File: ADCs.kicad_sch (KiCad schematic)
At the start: 4 parts, among them U3 ADS7828, U4 ADS7828

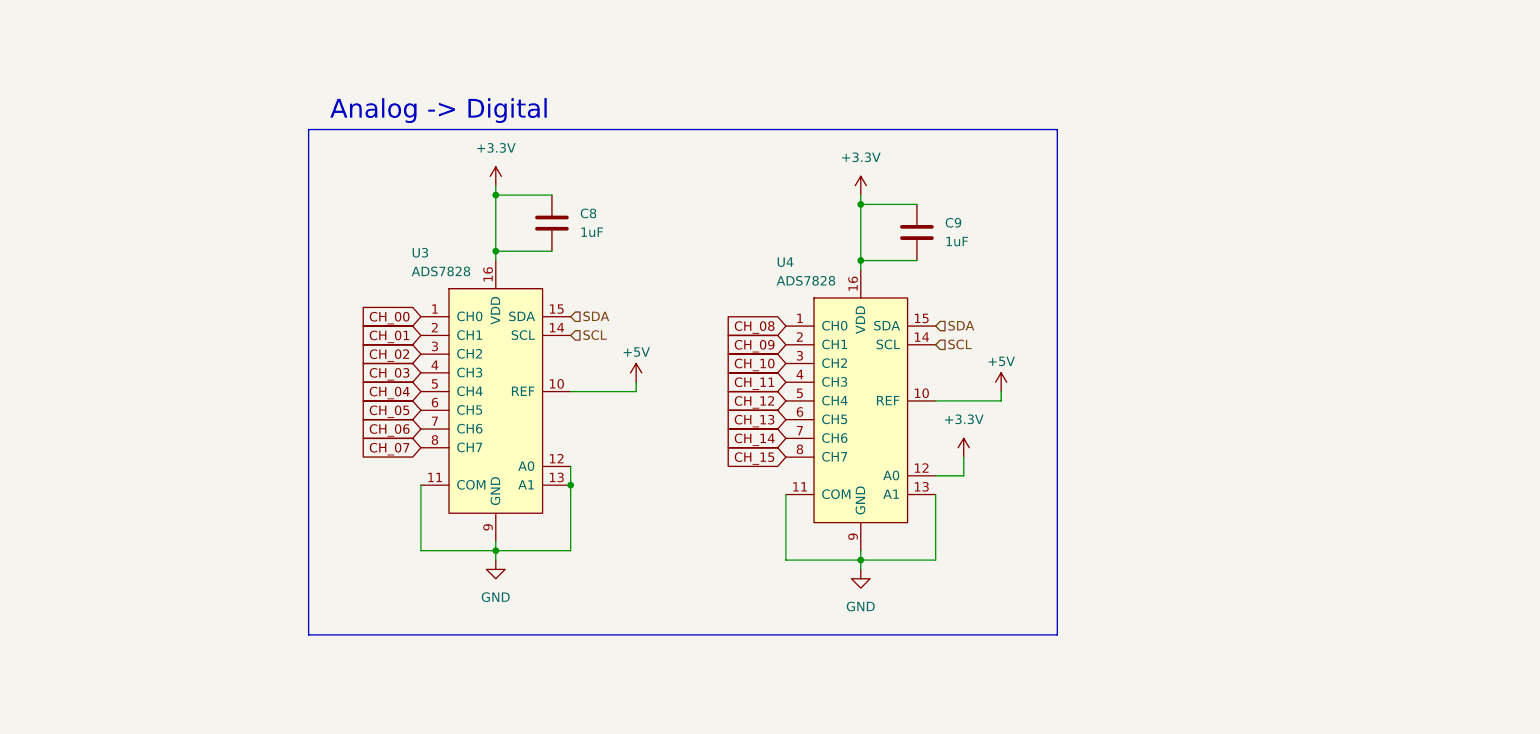
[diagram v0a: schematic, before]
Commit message: layout🏄‍♂️
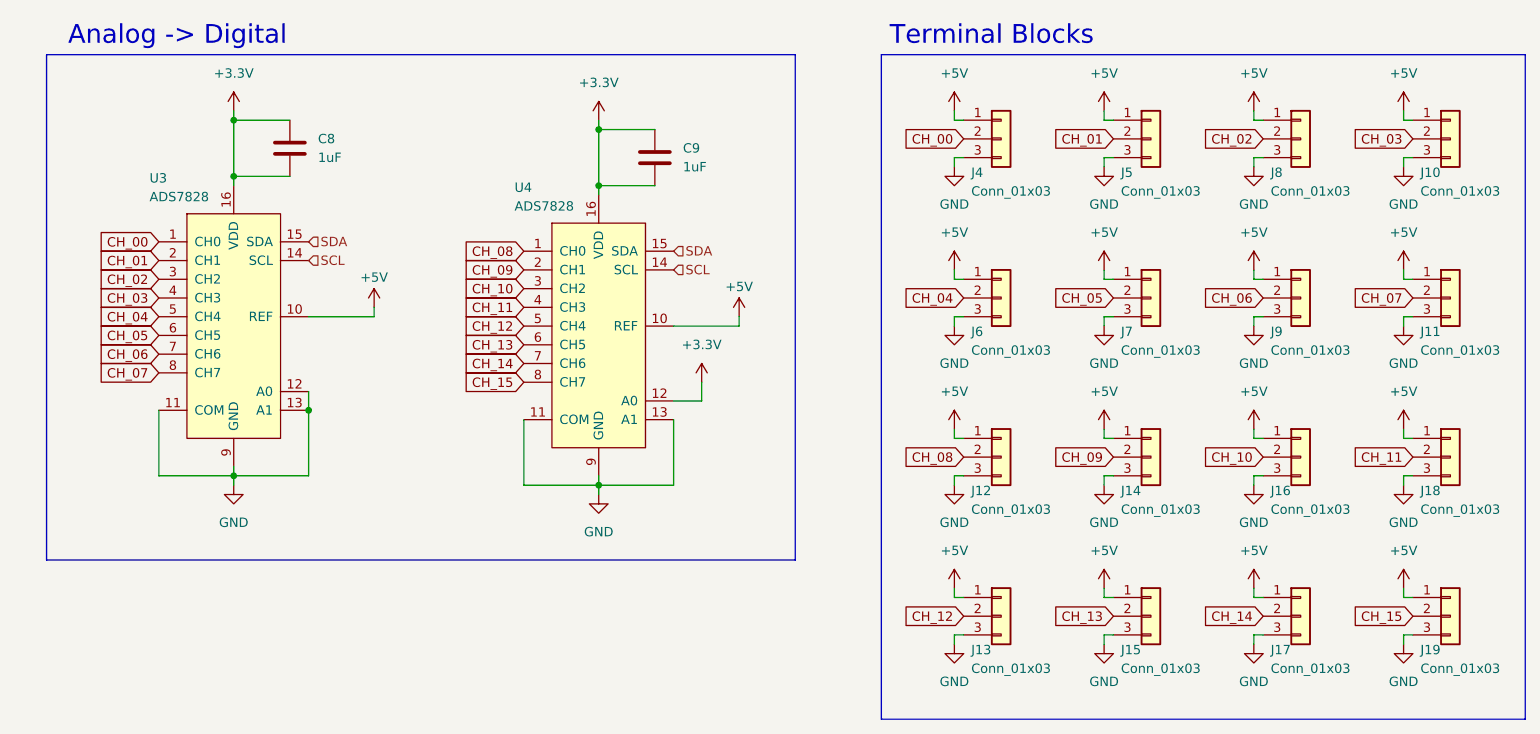
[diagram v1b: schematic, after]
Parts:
- added J10, J11, J12, J13, J14, J15, J16, J17, J18, J19, J4, J5, J6, J7, J8, J9: Conn_01x03, TerminalBlock_Phoenix:TerminalBlock_Phoenix_MPT-0,5-3-2.54_1x03_P2.54mm_Horizontal, symbol Connector_Generic:Conn_01x03
- C8, C9: footprint (none) -> Capacitor_SMD:C_0603_1608Metric
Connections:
- net +5V: now also J10.1 (Pin_1), J11.1 (Pin_1), J12.1 (Pin_1), J13.1 (Pin_1), J14.1 (Pin_1), J15.1 (Pin_1), J16.1 (Pin_1), J17.1 (Pin_1), J18.1 (Pin_1), J19.1 (Pin_1), J4.1 (Pin_1), J5.1 (Pin_1), J6.1 (Pin_1), J7.1 (Pin_1), J8.1 (Pin_1), J9.1 (Pin_1)
- net CH_00: now also J4.2 (Pin_2)
- net CH_01: now also J5.2 (Pin_2)
- net CH_02: now also J8.2 (Pin_2)
- net CH_03: now also J10.2 (Pin_2)
- net CH_04: now also J6.2 (Pin_2)
- net CH_05: now also J7.2 (Pin_2)
- net CH_06: now also J9.2 (Pin_2)
- net CH_07: now also J11.2 (Pin_2)
- net CH_08: now also J12.2 (Pin_2)
- net CH_09: now also J14.2 (Pin_2)
- net CH_10: now also J16.2 (Pin_2)
- net CH_11: now also J18.2 (Pin_2)
- net CH_12: now also J13.2 (Pin_2)
- net CH_13: now also J15.2 (Pin_2)
- net CH_14: now also J17.2 (Pin_2)
- net CH_15: now also J19.2 (Pin_2)
- net GND: now also J10.3 (Pin_3), J11.3 (Pin_3), J12.3 (Pin_3), J13.3 (Pin_3), J14.3 (Pin_3), J15.3 (Pin_3), J16.3 (Pin_3), J17.3 (Pin_3), J18.3 (Pin_3), J19.3 (Pin_3), J4.3 (Pin_3), J5.3 (Pin_3), J6.3 (Pin_3), J7.3 (Pin_3), J8.3 (Pin_3), J9.3 (Pin_3)
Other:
- note added: "Terminal Blocks"
- moved on the sheet: C8, C9, U3, U4
